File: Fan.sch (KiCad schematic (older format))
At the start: 0 parts

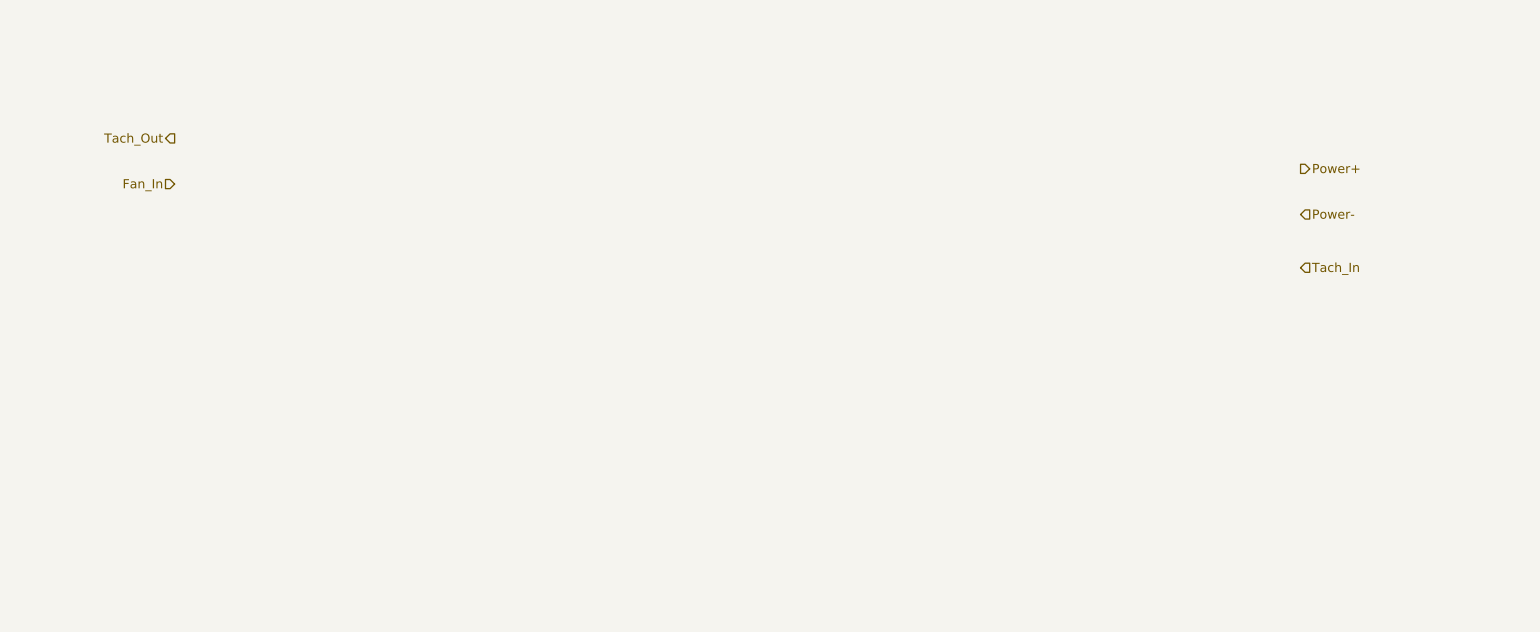
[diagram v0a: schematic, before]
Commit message: Understanding the Current/Fan Driver Module
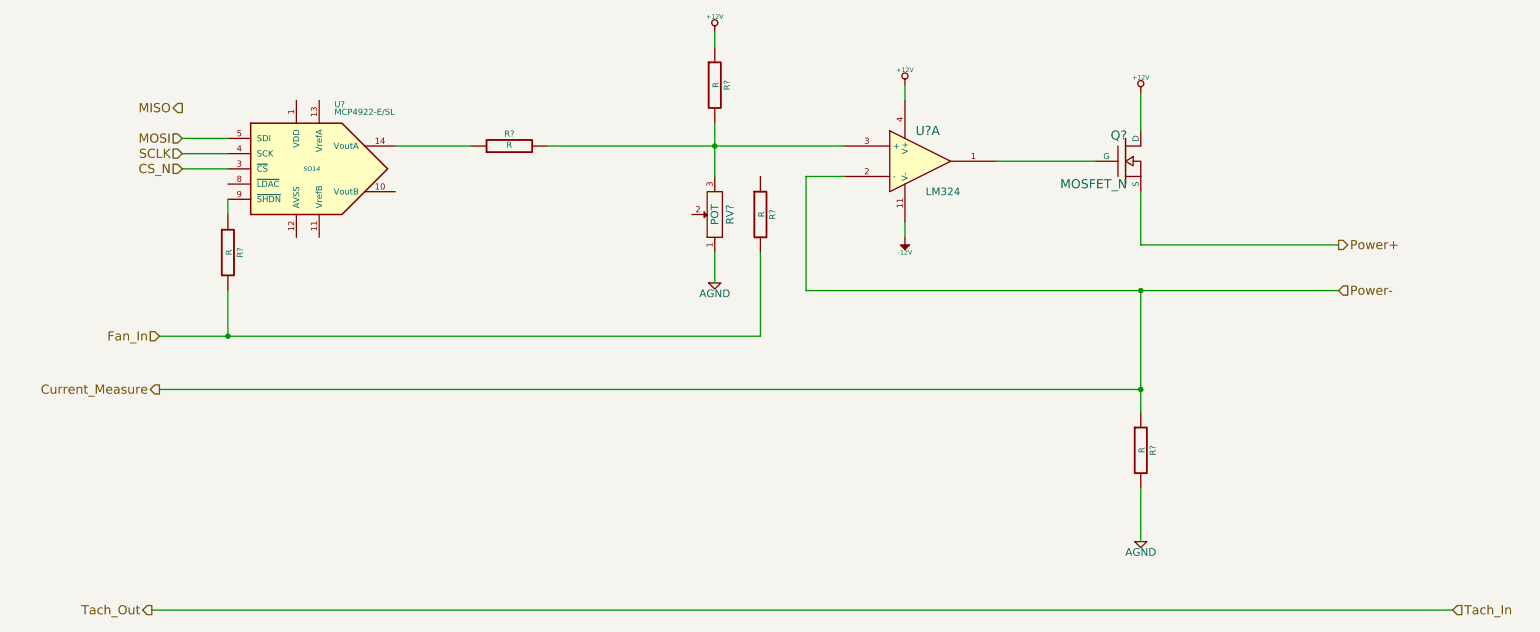
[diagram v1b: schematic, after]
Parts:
- added Q?: MOSFET_N, symbol MOSFET_N
- added R? (x5): R, symbol R
- added RV?: POT, symbol POT
- added U?: LM324, symbol LM324
- added U?: MCP4922-E/SL, SO14, symbol MCP4922-E/SL
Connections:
- net Fan_In: now also R?.2, R?.2
- net Power+: now also Q?.S
- new net: Q?.G, U?.1
- new net: R?.2, R?.2, RV?.3, U?.3 (+)
- new net: R?.1, U?.14 (VoutA)
- new net: R?.1, U?.9 (~SHDN~)
- new net +12V: Q?.D, R?.1, U?.4 (V+)
- new net -12V: U?.11 (V-)
- new net AGND: R?.2, RV?.1
- new net CS_N: U?.3 (~CS~)
- new net Current_Measure: R?.1, U?.2 (-)
- new net MOSI: U?.5 (SDI)
- new net SCLK: U?.4 (SCK)
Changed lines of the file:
@@
 LIBS:contrib
 LIBS:valves
+LIBS:MyComponents
 LIBS:BenchBuddy-cache
 EELAYER 24 0
@@
 Comment4 ""
 $EndDescr
-Text HLabel 9250 2250 2    60   Output ~ 0
+Text HLabel 9500 2750 2    60   Output ~ 0
 Power+
-Text HLabel 9250 2550 2    60   Input ~ 0
+Text HLabel 9500 3050 2    60   Input ~ 0
 Power-
-Text HLabel 9250 2900 2    60   Input ~ 0
+Text HLabel 10250 5150 2    60   Input ~ 0
 Tach_In
-Text HLabel 1850 2050 0    60   Output ~ 0
+Text HLabel 1700 5150 0    60   Output ~ 0
 Tach_Out
-Text HLabel 1850 2350 0    60   Input ~ 0
+Text HLabel 1750 3350 0    60   Input ~ 0
 Fan_In
+Wire Wire Line
+	1700 5150 10250 5150
+$Comp
+L LM324 U?
+U 1 1 52F15AC1
+P 6750 2200
+F 0 "U?" H 6800 2400 60  0000 C CNN
+F 1 "LM324" H 6900 2000 50  0000 C CNN
+F 2 "" H 6750 2200 60  0000 C CNN
+F 3 "" H 6750 2200 60  0000 C CNN
+	1    6750 2200
+	1    0    0    -1
+$EndComp
+$Comp
+L MOSFET_N Q?
+U 1 1 52F15ADF
+P 8100 2200
+F 0 "Q?" H 8110 2370 60  0000 R CNN
+F 1 "MOSFET_N" H 8110 2050 60  0000 R CNN
+F 2 "" H 8100 2200 60  0000 C CNN
+F 3 "" H 8100 2200 60  0000 C CNN
+	1    8100 2200
+	1    0    0    -1
+$EndComp
+$Comp
+L +12V #PWR?
+U 1 1 52F15AF3
+P 8200 1750
+F 0 "#PWR?" H 8200 1700 20  0001 C CNN
+F 1 "+12V" H 8200 1850 30  0000 C CNN
+F 2 "" H 8200 1750 60  0000 C CNN
+F 3 "" H 8200 1750 60  0000 C CNN
+	1    8200 1750
+	1    0    0    -1
+$EndComp
+Wire Wire Line
+	7900 2200 7250 2200
+Wire Wire Line
+	8200 2400 8200 2750
+Wire Wire Line
+	8200 2750 9500 2750
+Wire Wire Line
+	6000 3050 9500 3050
+Wire Wire Line
+	8200 3050 8200 3850
+$Comp
+L R R?
+U 1 1 52F15B2A
+P 8200 4100
+F 0 "R?" V 8280 4100 40  0000 C CNN
+F 1 "R" V 8207 4101 40  0000 C CNN
+F 2 "" V 8130 4100 30  0000 C CNN
+F 3 "" H 8200 4100 30  0000 C CNN
+	1    8200 4100
+	1    0    0    -1
+$EndComp
+$Comp
+L AGND #PWR?
+U 1 1 52F15B46
+P 8200 4700
+F 0 "#PWR?" H 8200 4700 40  0001 C CNN
+F 1 "AGND" H 8200 4630 50  0000 C CNN
+F 2 "" H 8200 4700 60  0000 C CNN
+F 3 "" H 8200 4700 60  0000 C CNN
+	1    8200 4700
+	1    0    0    -1
+$EndComp
+Wire Wire Line
+	8200 4350 8200 4700
+Wire Wire Line
+	6000 3050 6000 2300
+Wire Wire Line
+	6000 2300 6250 2300
+Connection ~ 8200 3050
+Wire Wire Line
+	8200 2000 8200 1750
+$Comp
+L +12V #PWR?
+U 1 1 52F15B77
+P 6650 1700
+F 0 "#PWR?" H 6650 1650 20  0001 C CNN
+F 1 "+12V" H 6650 1800 30  0000 C CNN
+F 2 "" H 6650 1700 60  0000 C CNN
+F 3 "" H 6650 1700 60  0000 C CNN
+	1    6650 1700
+	1    0    0    -1
+$EndComp
+Wire Wire Line
+	6650 1700 6650 1800
+$Comp
+L -12V #PWR?
+U 1 1 52F15B91
+P 6650 2700
+F 0 "#PWR?" H 6650 2830 20  0001 C CNN
+F 1 "-12V" H 6650 2800 30  0000 C CNN
+F 2 "" H 6650 2700 60  0000 C CNN
+F 3 "" H 6650 2700 60  0000 C CNN
+	1    6650 2700
+	-1   0    0    1
+$EndComp
+Wire Wire Line
+	6650 2700 6650 2600
+$Comp
+L R R?
+U 1 1 52F15BC1
+P 5400 1700
+F 0 "R?" V 5480 1700 40  0000 C CNN
+F 1 "R" V 5407 1701 40  0000 C CNN
+F 2 "" V 5330 1700 30  0000 C CNN
+F 3 "" H 5400 1700 30  0000 C CNN
+	1    5400 1700
+	1    0    0    -1
+$EndComp
+$Comp
+L +12V #PWR?
+U 1 1 52F15BCC
+P 5400 1350
+F 0 "#PWR?" H 5400 1300 20  0001 C CNN
+F 1 "+12V" H 5400 1450 30  0000 C CNN
+F 2 "" H 5400 1350 60  0000 C CNN
+F 3 "" H 5400 1350 60  0000 C CNN
+	1    5400 1350
+	1    0    0    -1
+$EndComp
+Wire Wire Line
+	5400 1350 5400 1450
+$Comp
+L POT RV?
+U 1 1 52F15C37
+P 5400 2550
+F 0 "RV?" H 5400 2450 50  0000 C CNN
+F 1 "POT" H 5400 2550 50  0000 C CNN
+F 2 "" H 5400 2550 60  0000 C CNN
+F 3 "" H 5400 2550 60  0000 C CNN
+	1    5400 2550
+	0    -1   -1   0
+$EndComp
+$Comp
+L AGND #PWR?
+U 1 1 52F15C5C
+P 5400 3000
+F 0 "#PWR?" H 5400 3000 40  0001 C CNN
+F 1 "AGND" H 5400 2930 50  0000 C CNN
+F 2 "" H 5400 3000 60  0000 C CNN
+F 3 "" H 5400 3000 60  0000 C CNN
+	1    5400 3000
+	1    0    0    -1
+$EndComp
+Wire Wire Line
+	5400 3000 5400 2800
+Wire Wire Line
+	5400 1950 5400 2300
+Wire Wire Line
+	4300 2100 6250 2100
+Connection ~ 5400 2100
+Text HLabel 1900 1850 0    60   Output ~ 0
+MISO
+Text HLabel 1900 2050 0    60   Input ~ 0
+MOSI
+Text HLabel 1900 2150 0    60   Input ~ 0
+SCLK
+Text HLabel 1900 2250 0    60   Input ~ 0
+CS_N
+Text HLabel 1750 3700 0    60   Output ~ 0
+Current_Measure
+$Comp
+L R R?
+U 1 1 52F15DC9
+P 5700 2550
+F 0 "R?" V 5780 2550 40  0000 C CNN
+F 1 "R" V 5707 2551 40  0000 C CNN
+F 2 "" V 5630 2550 30  0000 C CNN
+F 3 "" H 5700 2550 30  0000 C CNN
+	1    5700 2550
+	1    0    0    -1
+$EndComp
+Wire Wire Line
+	1750 3700 8200 3700
+Connection ~ 8200 3700
+Wire Wire Line
+	5700 3350 5700 2800
+Wire Wire Line
+	1750 3350 5700 3350
+$Comp
+L R R?
+U 1 1 52F15E21
+P 4050 2100
+F 0 "R?" V 4130 2100 40  0000 C CNN
+F 1 "R" V 4057 2101 40  0000 C CNN
+F 2 "" V 3980 2100 30  0000 C CNN
+F 3 "" H 4050 2100 30  0000 C CNN
+	1    4050 2100
+	0    -1   -1   0
+$EndComp
+Wire Wire Line
+	1900 2050 2200 2050
+Wire Wire Line
+	1900 2150 2200 2150
+Wire Wire Line
+	1900 2250 2200 2250
+$Comp
+L R R?
+U 1 1 52F15EBA
+P 2200 2800
+F 0 "R?" V 2280 2800 40  0000 C CNN
+F 1 "R" V 2207 2801 40  0000 C CNN
+F 2 "" V 2130 2800 30  0000 C CNN
+F 3 "" H 2200 2800 30  0000 C CNN
+	1    2200 2800
+	1    0    0    -1
+$EndComp
+Wire Wire Line
+	2200 3050 2200 3350
+Connection ~ 2200 3350
+$Comp
+L MCP4922-E/SL U?
+U 1 1 52F15F05
+P 2750 2250
+F 0 "U?" H 2900 2650 40  0000 L BNN
+F 1 "MCP4922-E/SL" H 2900 2600 40  0000 L BNN
+F 2 "SO14" H 2750 2250 30  0000 C CIN
+F 3 "" H 2750 2250 60  0000 C CNN
+	1    2750 2250
+	1    0    0    -1
+$EndComp
+Wire Wire Line
+	3300 2100 3800 2100
+Wire Wire Line
+	2200 2450 2200 2550
 $EndSCHEMATC
